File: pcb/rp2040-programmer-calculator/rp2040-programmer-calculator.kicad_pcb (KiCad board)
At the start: 2 copper layers, 105 x 205 mm, 281 parts, among them J1 5*2.54mm DNP, J2 USB4105-GF-A, Q1 AO3401A, Q2 BSS84, Q3 MMBT3904, Q4 DMG1012T, SW1 PTS636SL50 LFS, SW10 PTS636SL50 LFS, SW11 PTS636SL50 LFS, SW12 PTS636SL50 LFS, SW13 PTS636SL50 LFS, SW14 PTS636SL50 LFS, SW15 PTS636SL50 LFS, SW16 PTS636SL50 LFS, SW17 PTS636SL50 LFS, SW18 PTS636SL50 LFS, SW19 PTS636SL50 LFS, SW2 PTS636SL50 LFS, SW20 PTS636SL50 LFS, SW21 PTS636SL50 LFS, SW22 PTS636SL50 LFS, SW23 PTS636SL50 LFS, SW24 PTS636SL50 LFS, SW25 PTS636SL50 LFS, SW26 PTS636SL50 LFS, SW27 PTS636SL50 LFS, SW28 PTS636SL50 LFS, SW29 PTS636SL50 LFS, SW3 PTS636SL50 LFS, SW30 PTS636SL50 LFS, SW31 PTS636SL50 LFS, SW32 PTS636SL50 LFS, SW33 PTS636SL50 LFS, SW34 B3F, SW35 B3F, SW36 B3F, SW37 B3F, SW38 B3F, SW39 B3F, SW4 PTS636SL50 LFS, SW40 B3F, SW41 B3F, SW42 B3F, SW43 B3F, SW44 B3F, SW45 B3F, SW46 B3F, SW47 B3F, SW48 B3F, SW49 B3F, SW5 PTS636SL50 LFS, SW50 B3F, SW51 B3F, SW52 B3F, SW53 B3F, SW54 B3F, SW55 B3F, SW56 B3F, SW57 B3F, SW58 B3F, SW59 B3F, SW6 PTS636SL50 LFS, SW60 B3F, SW61 B3F, SW62 B3F, SW63 B3F, SW64 PTS636SL50 LFS, SW7 PTS636SL50 LFS, SW8 PTS636SL50 LFS, SW9 PTS636SL50 LFS, U1 RP2040, U10 XB7608AJ, U11 3.12" SSD1322 OLED, U2 TCA8418RTWR, U3 74HC595, U4 74HC595, U5 74HC595, U6 74HC595, U7 W25Q32JVSS, U8 TP4057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

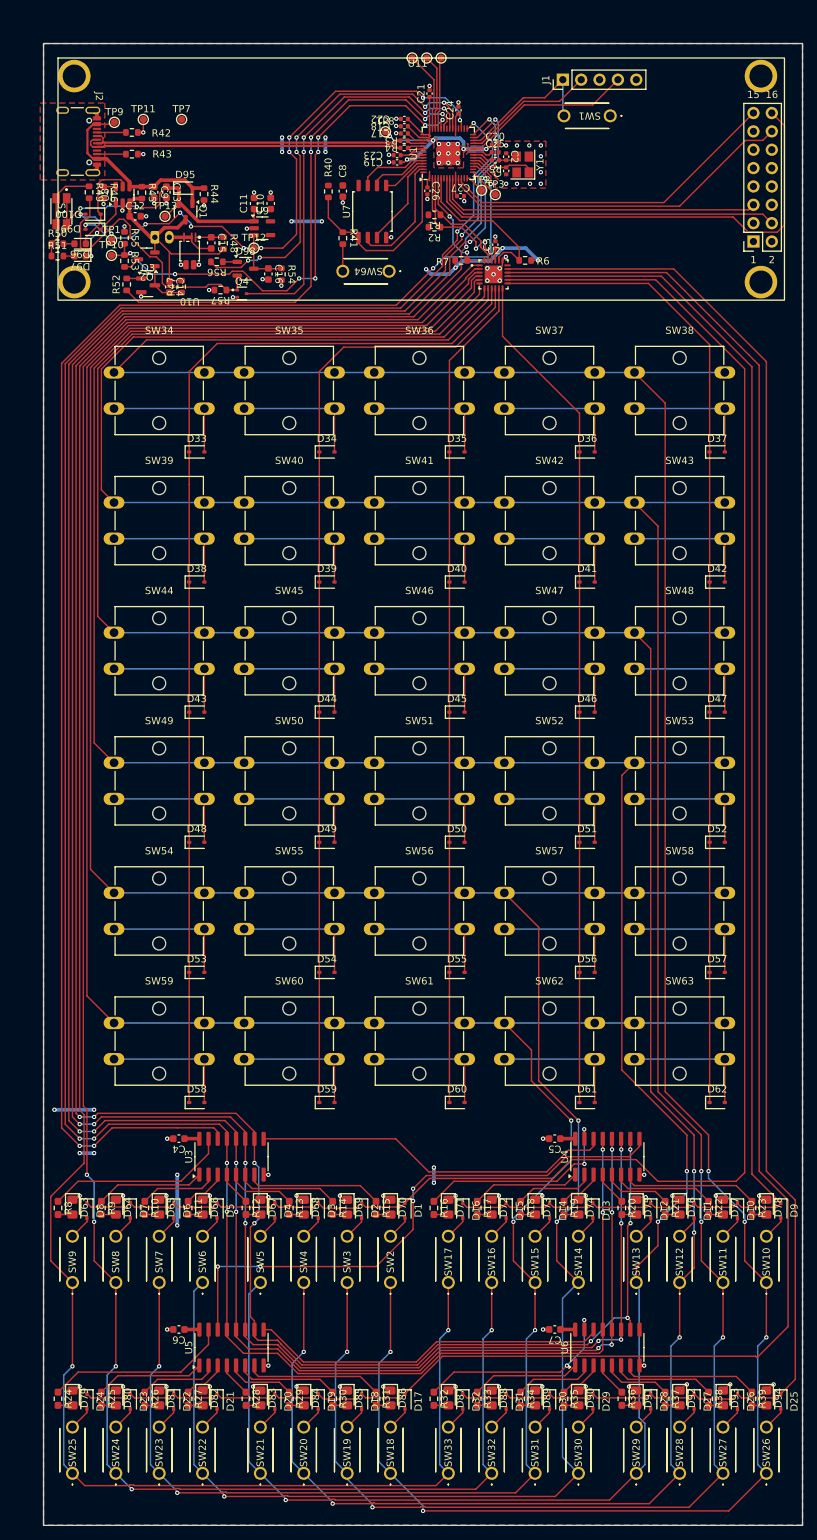
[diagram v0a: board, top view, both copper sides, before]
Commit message: Finished design
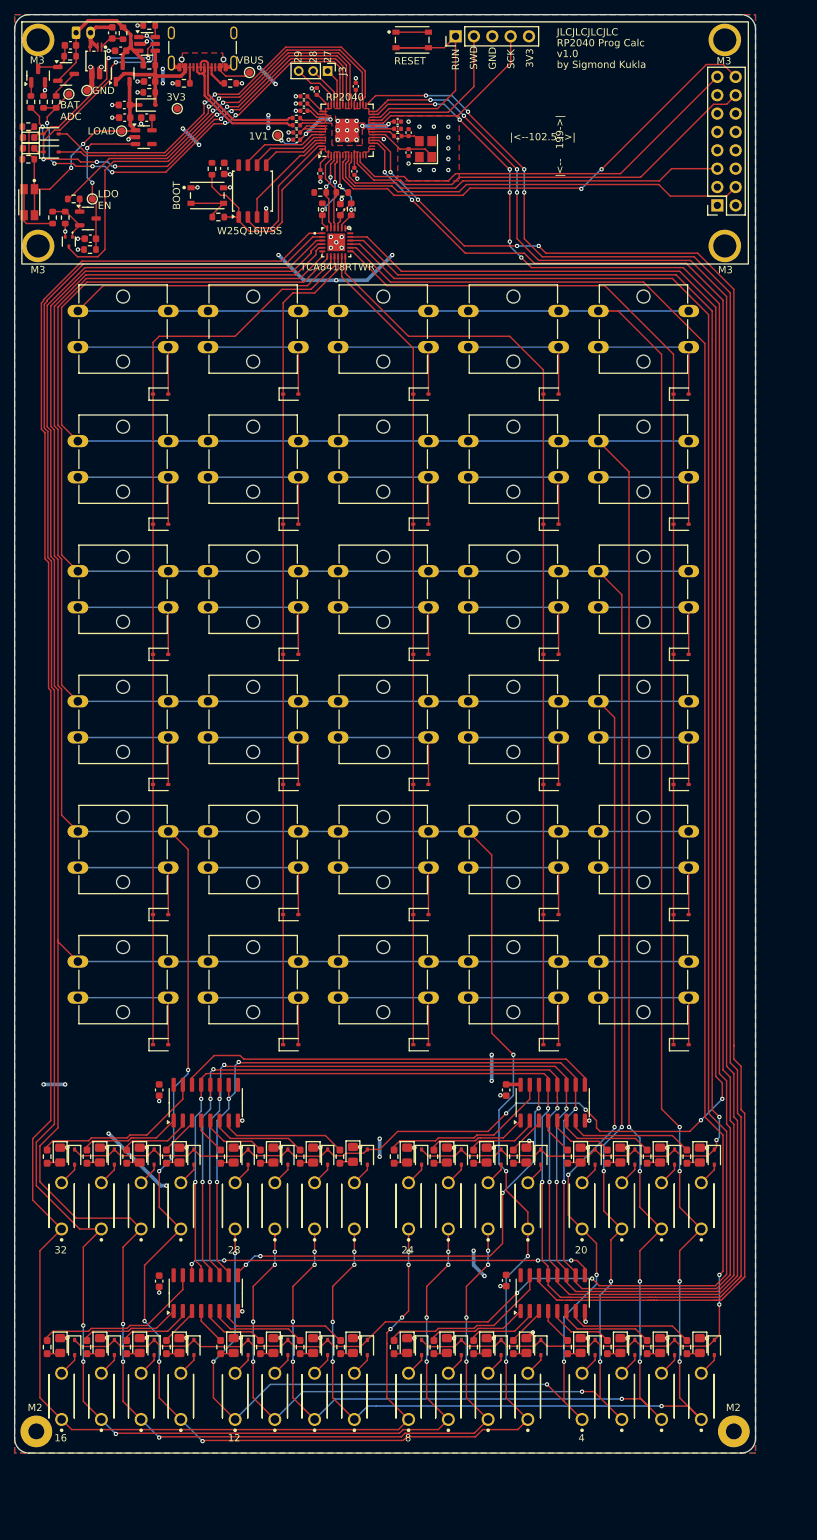
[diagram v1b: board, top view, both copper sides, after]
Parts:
- removed S1: EVQ-P7A01P, SamacSys_Parts:EVQP7J01P
- removed SW64: PTS636SL50 LFS, SamacSys_Parts:PTS636SL50LFS
- removed TP1: ~{STDBY}, TestPoint:TestPoint_Pad_D1.0mm
- removed TP2: GPIO11, TestPoint:TestPoint_Pad_D1.0mm
- removed TP3: GPIO12, TestPoint:TestPoint_Pad_D1.0mm
- removed TP4: GPIO27, TestPoint:TestPoint_Pad_D1.0mm
- removed TP5: GPIO28, TestPoint:TestPoint_Pad_D1.0mm
- removed TP6: GPIO29, TestPoint:TestPoint_Pad_D1.0mm
- added J3: Spare GPIO, Connector_PinHeader_2.00mm:PinHeader_1x03_P2.00mm_Vertical, F.Cu at (57.3, 21.8)
- added REF**: MountingHole_2.2mm_M2_Pad, MountingHole:MountingHole_2.2mm_M2_Pad, F.Cu at (17.0, 210.0)
- added REF**: MountingHole_2.2mm_M2_Pad, MountingHole:MountingHole_2.2mm_M2_Pad, F.Cu at (113.5, 210.0)
- added SW65: EVQ-P7A01P, EVQP7J01P:EVQP7J01P, F.Cu at (16.0, 39.6)
- added SW66: PTS815_SJM_250_SMTR_LFS, PTS815_SJM_250_SMTR_LFS:SW_Push_PTS815_SJM_250_SMTR_LFS, F.Cu at (40.6, 39.0)
- BT1: footprint Connector_JST:JST_PH_S2B-PH-K_1x02_P2.00mm_Horizontal_Reverse_Polarity -> JST_PH_S2B_Reverse_Polarity:JST_PH_S2B-PH-K_1x02_P2.00mm_Horizontal
- C15: value 0.1u -> 100n
- C3: footprint Capacitor_SMD:C_0402_1005Metric -> Capacitor_SMD:C_0603_1608Metric
- SW1: value PTS636SL50 LFS -> PTS815_SJM_250_SMTR_LFS; footprint SamacSys_Parts:PTS636SL50LFS -> PTS815_SJM_250_SMTR_LFS:SW_Push_PTS815_SJM_250_SMTR_LFS
- SW10, SW11, SW12, SW13, SW14, SW15, SW16, SW17, SW18, SW19, SW2, SW20, SW21, SW22, SW23, SW24, SW25, SW26, SW27, SW28, SW29, SW3, SW30, SW31, SW32, SW33, SW4, SW5, SW6, SW7, SW8, SW9: footprint SamacSys_Parts:PTS636SL50LFS -> PTS636SL50LFS:PTS636SL50LFS
- U2: footprint TCA8418RWTR:QFN50P400X400X80-25N -> TCA8418RTWR:QFN50P400X400X80-25N
- U7: value W25Q32JVSS -> W25Q16JVSS; footprint Package_SO:SOIC-8_5.23x5.23mm_P1.27mm -> Package_SO:SOIC-8_5.3x5.3mm_P1.27mm
- moved D94 103.3 mm to (20.3, 171.8)
- moved R39 103.1 mm to (18.5, 172.0)
- moved D78 99.6 mm to (20.3, 198.1)
- moved R23 99.4 mm to (18.5, 198.3)
- moved R24 93.2 mm to (107.0, 172.0)
- moved D79 93.1 mm to (108.8, 171.8)
- moved D93 92.5 mm to (25.8, 171.8)
- moved R38 92.3 mm to (24.0, 172.0)
- moved R8 89.1 mm to (107.0, 198.3)
- moved D63 88.9 mm to (108.8, 198.1)
- moved D77 88.3 mm to (25.8, 198.1)
- moved R22 88.1 mm to (24.0, 198.3)
- moved R25 82.6 mm to (101.5, 172.0)
- moved D80 82.5 mm to (103.3, 171.8)
- moved D92 81.9 mm to (31.3, 171.8)
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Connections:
- net /Bit LEDs/LED_Byte_3/QH' renamed /Bit LEDs/LED_Byte_3/QH&apos;
- D100 pad 2: /Power/~{STDBY} -> /~{STDBY}
- R10 pad 1: Net-(U3-QC) -> Net-(U3-QF)
- R11 pad 1: Net-(U3-QD) -> Net-(U3-QE)
- R12 pad 1: Net-(U3-QE) -> Net-(U3-QD)
- R13 pad 1: Net-(U3-QF) -> Net-(U3-QC)
- R14 pad 1: Net-(U3-QG) -> Net-(U3-QB)
- R15 pad 1: Net-(U3-QH) -> Net-(U3-QA)
- R16 pad 1: Net-(U4-QA) -> Net-(U4-QH)
- R17 pad 1: Net-(U4-QB) -> Net-(U4-QG)
- R18 pad 1: Net-(U4-QC) -> Net-(U4-QF)
- R19 pad 1: Net-(U4-QD) -> Net-(U4-QE)
- R20 pad 1: Net-(U4-QE) -> Net-(U4-QD)
- R21 pad 1: Net-(U4-QF) -> Net-(U4-QC)
- R22 pad 1: Net-(U4-QG) -> Net-(U4-QB)
- R23 pad 1: Net-(U4-QH) -> Net-(U4-QA)
- R24 pad 1: Net-(U5-QA) -> Net-(U5-QH)
- R25 pad 1: Net-(U5-QB) -> Net-(U5-QG)
- R26 pad 1: Net-(U5-QC) -> Net-(U5-QF)
- R27 pad 1: Net-(U5-QD) -> Net-(U5-QE)
- R28 pad 1: Net-(U5-QE) -> Net-(U5-QD)
- R29 pad 1: Net-(U5-QF) -> Net-(U5-QC)
- R30 pad 1: Net-(U5-QG) -> Net-(U5-QB)
- R31 pad 1: Net-(U5-QH) -> Net-(U5-QA)
- R32 pad 1: Net-(U6-QA) -> Net-(U6-QH)
- R33 pad 1: Net-(U6-QB) -> Net-(U6-QG)
- R34 pad 1: Net-(U6-QC) -> Net-(U6-QF)
- R35 pad 1: Net-(U6-QD) -> Net-(U6-QE)
- R36 pad 1: Net-(U6-QE) -> Net-(U6-QD)
- R37 pad 1: Net-(U6-QF) -> Net-(U6-QC)
- R38 pad 1: Net-(U6-QG) -> Net-(U6-QB)
- R39 pad 1: Net-(U6-QH) -> Net-(U6-QA)
- R8 pad 1: Net-(U3-QA) -> Net-(U3-QH)
- R9 pad 1: Net-(U3-QB) -> Net-(U3-QG)
- U1 pad 14: Net-(U1-GPIO11) -> unconnected-(U1-GPIO11-Pad14)
- U1 pad 15: Net-(U1-GPIO12) -> unconnected-(U1-GPIO12-Pad15)
- U1 pad 30: unconnected-(U1-GPIO19-Pad30) -> /~{STDBY}
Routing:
- net /Matrix/C6: track 203.6 -> 287.4 mm, vias 0 -> 2
- net /Matrix/C7: track 279.2 -> 216.5 mm, vias 0 -> 2
- net /~{STDBY}: track 0.00 -> 56.6 mm, vias 0 -> 2
- net /Matrix/R4: track 389.3 -> 429.1 mm, vias 3 -> 9
- net Net-(Q4-G): track 40.0 -> 6.55 mm
- net /Matrix/C8: track 233.8 -> 265.9 mm, vias 0 -> 4
- net /USB/USB_DN: track 44.5 -> 19.5 mm
- net /Matrix/R1: track 386.4 -> 361.7 mm, vias 5 -> 9
- net /USB/USB_DP: track 44.6 -> 20.3 mm
- net /~{CHRG}: track 78.6 -> 54.7 mm, vias 10 -> 2
- net /Matrix/R2: track 385.1 -> 361.5 mm, vias 5 -> 9
- net /Matrix/R3: track 389.1 -> 366.0 mm, vias 3 -> 7
- net /Matrix/R0: track 386.9 -> 364.8 mm, vias 5 -> 9
- net /Matrix/C0: track 149.0 -> 128.0 mm
- net /LED_SER: track 210.2 -> 229.9 mm
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- added copper zone on F.Cu, net VBUS
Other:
- board size 105 x 205 mm -> 102.5 x 199 mm
- board text added: "- +"
- board text added: "12"
- board text added: "16"
- board text added: "1V1"
- board text added: "20"
- board text added: "24"
- board text added: "27"
- board text added: "28"
- board text added: "29"
- board text added: "3.7V"
- board text added: "32"
- board text added: "3V3"
- board text added: "4"
- board text added: "8"
- board text added: "BAT ADC"
- board text added: "BOOT"
- board text added: "CHRG"
- board text added: "GND"
- board text added: "JLCJLCJLCJLC"
- board text added: "LDO EN"
- board text added: "LOAD"
- board text added: "M2"
- board text added: "M3"
- board text added: "POWER"
- board text added: "RESET"
- board text added: "RP2040"
- board text added: "RP2040 Prog Calc"
- board text added: "RUN"
- board text added: "SCK"
- board text added: "STDBY"
- board text added: "SWD"
- board text added: "TCA8418RTWR"
- board text added: "VBUS"
- board text added: "W25Q16JVSS"
- board text added: "by Sigmond Kukla"
- board text added: "v1.0"
- board text added: "|<-- 199->|"
- board text added: "|<--102.5-->|"
